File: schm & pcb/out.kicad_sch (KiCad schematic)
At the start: 11 parts

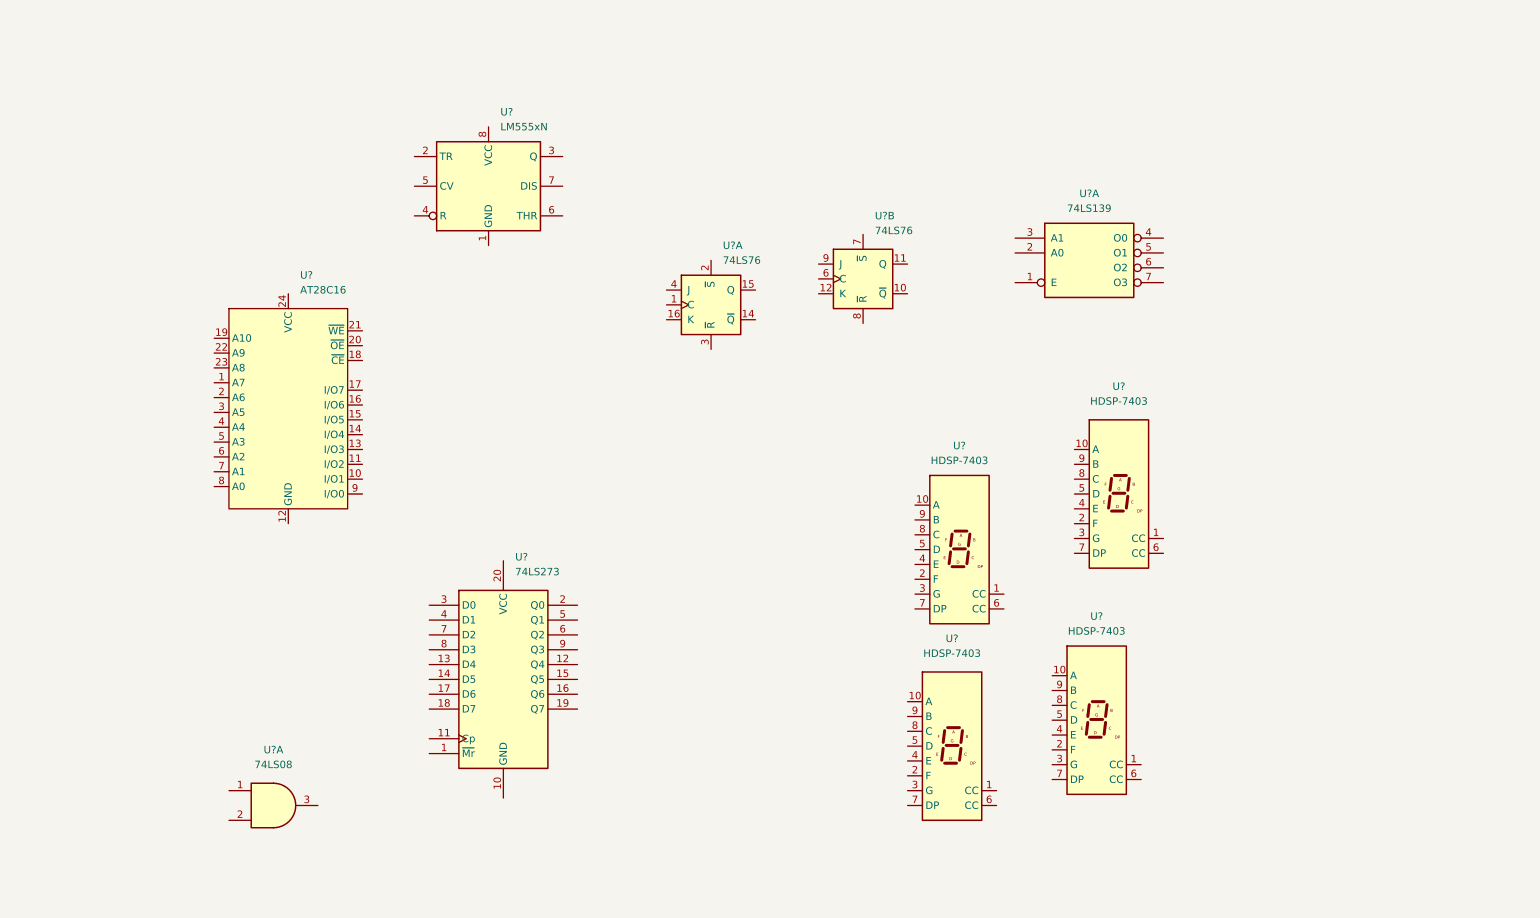
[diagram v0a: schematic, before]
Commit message: update from mac
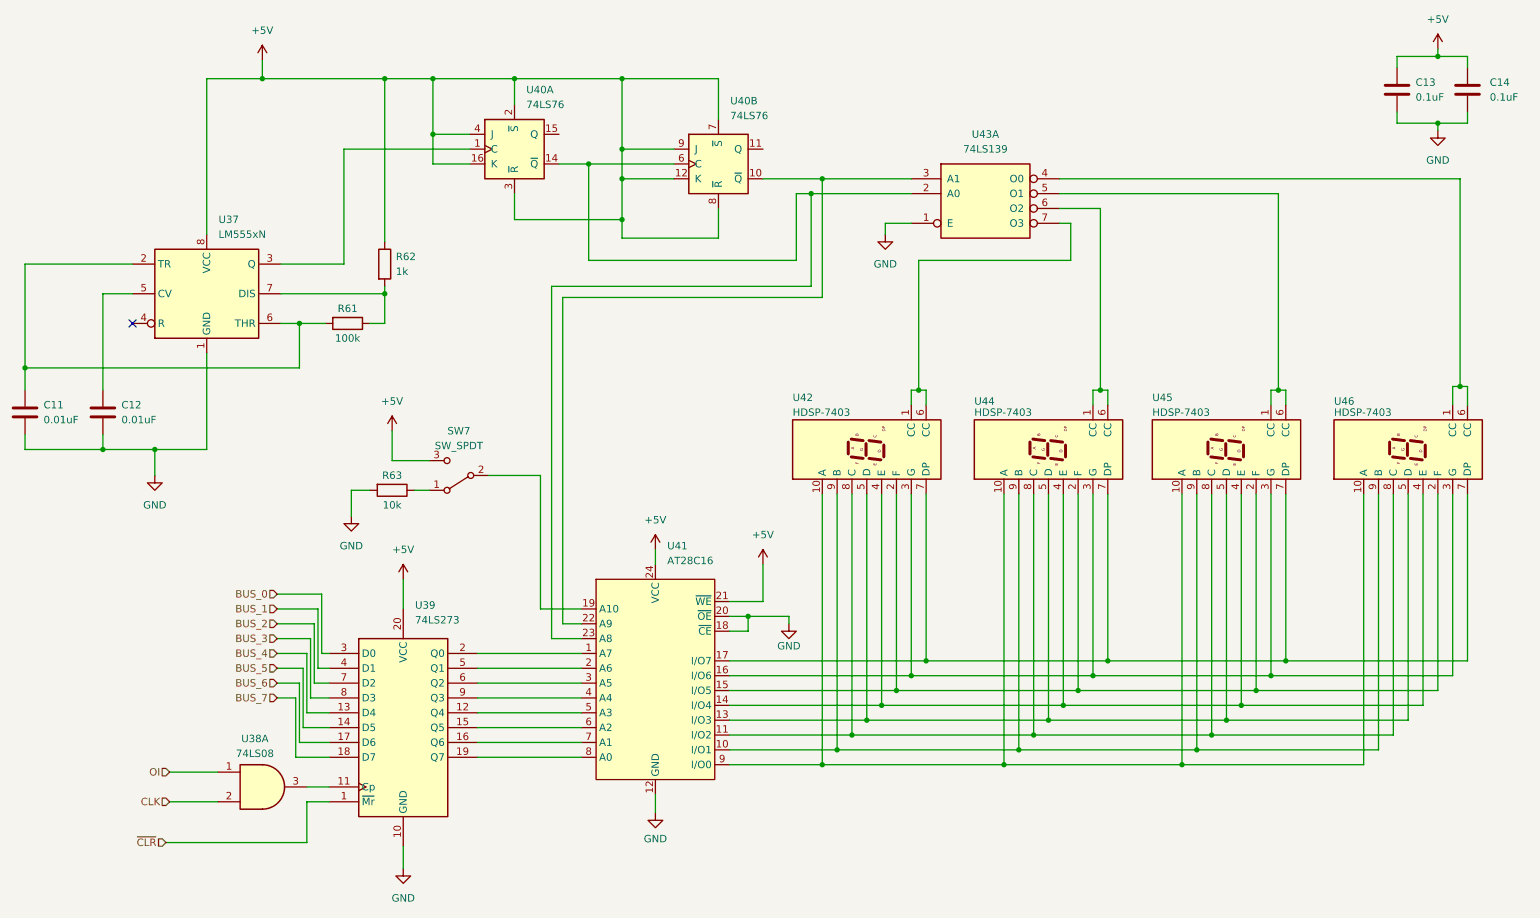
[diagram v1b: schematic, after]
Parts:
- added C11, C12: 0.01uF, symbol Device:C
- added C13, C14: 0.1uF, symbol Device:C
- added R61: 100k, symbol Device:R
- added R62: 1k, symbol Device:R
- added R63: 10k, symbol Device:R
- added SW7: SW_SPDT, symbol Switch:SW_SPDT
- gave numbers to parts that had none: 10
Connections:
- net at U41.1 (A7): now also U39.2 (Q0)
- net at U41.10 (I/O1): now also U42.9 (B), U44.9 (B), U45.9 (B), U46.9 (B)
- net at U41.11 (I/O2): now also U42.8 (C), U44.8 (C), U45.8 (C), U46.8 (C)
- net GND: now reaches U41.12 (GND)
- net GND: now also U37.1 (GND), U39.10 (GND), U41.18 (~{CE}), U41.20 (~{OE}), U43.1 (E), C11.2, C12.2, C13.2, C14.2, R63.2
- net at U41.13 (I/O3): now also U42.5 (D), U44.5 (D), U45.5 (D), U46.5 (D)
- net at U41.14 (I/O4): now also U42.4 (E), U44.4 (E), U45.4 (E), U46.4 (E)
- net at U41.15 (I/O5): now also U42.2 (F), U44.2 (F), U45.2 (F), U46.2 (F)
- net at U41.16 (I/O6): now also U42.3 (G), U44.3 (G), U45.3 (G), U46.3 (G)
- net at U41.17 (I/O7): now also U42.7 (DP), U44.7 (DP), U45.7 (DP), U46.7 (DP)
- net at U41.19 (A10): now also SW7.2 (B)
- net at U41.2 (A6): now also U39.5 (Q1)
- net +5V: now reaches U41.21 (~{WE})
- net +5V: now also U37.8 (VCC), U39.20 (VCC), U40.12 (K), U40.16 (K), U40.2 (~{S}), U40.3 (~{R}), U40.4 (J), U40.7 (~{S}), U40.8 (~{R}), U40.9 (J), U41.24 (VCC), C13.1, C14.1, R62.1, SW7.3 (C)
- net at U41.22 (A9): now also U40.10 (~{Q}), U43.3 (A1)
- net at U41.23 (A8): now also U40.14 (~{Q}), U40.6 (C), U43.2 (A0)
- net at U41.3 (A5): now also U39.6 (Q2)
- net at U41.4 (A4): now also U39.9 (Q3)
- net at U41.5 (A3): now also U39.12 (Q4)
- net at U41.6 (A2): now also U39.15 (Q5)
- net at U41.7 (A1): now also U39.16 (Q6)
- net at U41.8 (A0): now also U39.19 (Q7)
- net at U41.9 (I/O0): now also U42.10 (A), U44.10 (A), U45.10 (A), U46.10 (A)
- net at U44.1 (CC): now also U43.6 (O2), U44.6 (CC)
- net OI: now reaches U38.1
- net CLK: now reaches U38.2
- net at U38.3: now also U39.11 (Cp)
- net at U42.1 (CC): now also U42.6 (CC), U43.7 (O3)
- net at U46.1 (CC): now also U43.4 (O0), U46.6 (CC)
- net ~{CLR}: now reaches U39.1 (~{Mr})
- net BUS_4: now reaches U39.13 (D4)
- net BUS_5: now reaches U39.14 (D5)
- net BUS_6: now reaches U39.17 (D6)
- net BUS_7: now reaches U39.18 (D7)
- net BUS_0: now reaches U39.3 (D0)
- net BUS_1: now reaches U39.4 (D1)
- net BUS_2: now reaches U39.7 (D2)
- net BUS_3: now reaches U39.8 (D3)
- net at U37.2 (TR): now also U37.6 (THR), C11.1, R61.2
- net at U37.3 (Q): now also U40.1 (C)
- net at U37.5 (CV): now also C12.1
- net at U37.7 (DIS): now also R61.1, R62.2
- net at U43.5 (O1): now also U45.1 (CC), U45.6 (CC)
- new net: R63.1, SW7.1 (A)
- no-connect marks 0 -> 1
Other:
- moved on the sheet: U37, U38A, U39, U40A, U40B, U41, U42, U43A, U44, U45, U46
